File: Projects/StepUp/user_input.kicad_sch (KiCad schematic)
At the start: 1 part, among them U6 COM-09032

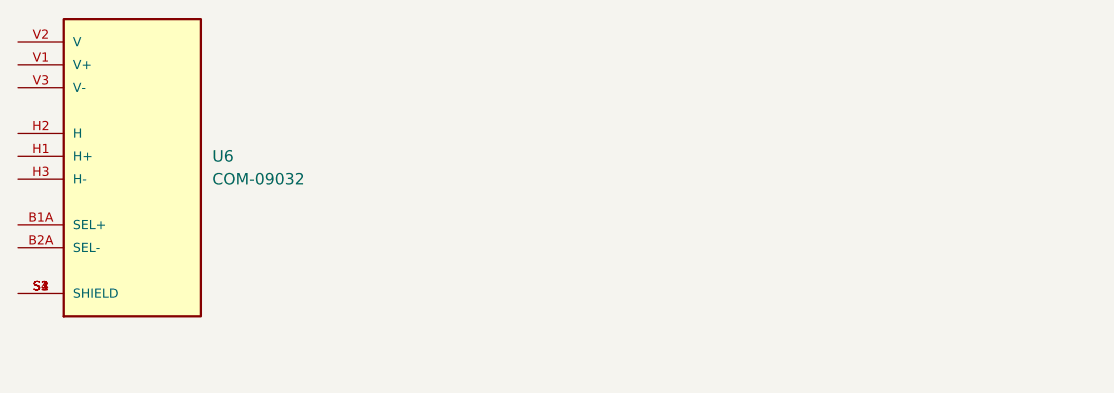
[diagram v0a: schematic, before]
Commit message: feat(charge): Charge IC, USB ESD, sheet sections
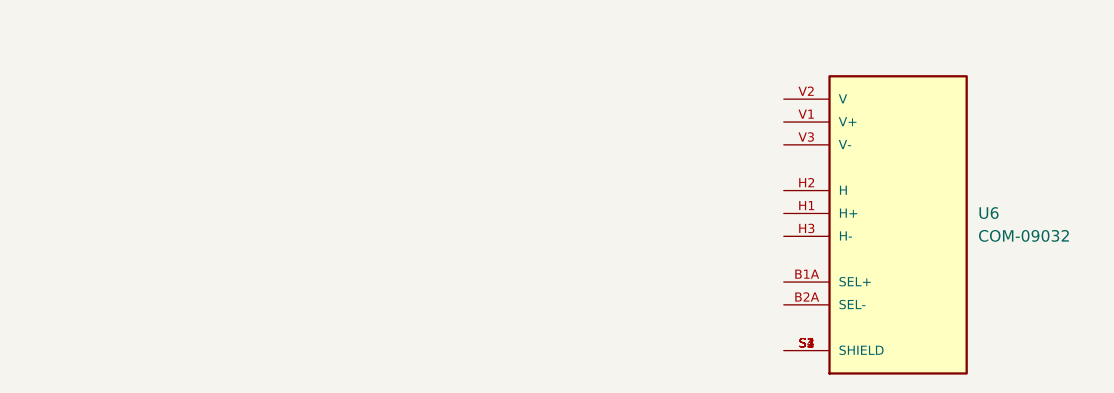
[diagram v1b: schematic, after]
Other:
- moved on the sheet: U6
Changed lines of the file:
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@@
 	(symbol
 		(lib_id "COM-09032:COM-09032")
-		(at 115.57 130.81 0)
+		(at 200.66 137.16 0)
 		(unit 1)
 		(exclude_from_sim no)
@@
 		(fields_autoplaced yes)
 		(property "Reference" "U6"
-			(at 124.46 130.8099 0)
+			(at 209.55 137.1599 0)
 			(effects
 				(font
@@
 		)
 		(property "Value" "COM-09032"
-			(at 124.46 133.3499 0)
+			(at 209.55 139.6999 0)
 			(effects
 				(font
@@
 		)
 		(property "Footprint" "joystick_footprints:XDCR_COM-09032"
-			(at 115.57 130.81 0)
+			(at 200.66 137.16 0)
 			(effects
 				(font
@@
 		)
 		(property "Datasheet" ""
-			(at 115.57 130.81 0)
+			(at 200.66 137.16 0)
 			(effects
 				(font
@@
 		)
 		(property "Description" ""
-			(at 115.57 130.81 0)
+			(at 200.66 137.16 0)
 			(effects
 				(font
@@
 		)
 		(property "MF" "SparkFun Electronics"
-			(at 115.57 130.81 0)
+			(at 200.66 137.16 0)
 			(effects
 				(font
@@
 		)
 		(property "MAXIMUM_PACKAGE_HEIGHT" "30.1mm"
-			(at 115.57 130.81 0)
+			(at 200.66 137.16 0)
 			(effects
 				(font
@@
 		)
 		(property "Package" "Package"
-			(at 115.57 130.81 0)
+			(at 200.66 137.16 0)
 			(effects
 				(font
@@
 		)
 		(property "Price" "None"
-			(at 115.57 130.81 0)
+			(at 200.66 137.16 0)
 			(effects
 				(font
@@
 		)
 		(property "Check_prices" "https://www.snapeda.com/parts/COM-09032/SparkFun+Electronics/view-part/?ref=eda"
-			(at 115.57 130.81 0)
+			(at 200.66 137.16 0)
 			(effects
 				(font
@@
 		)
 		(property "STANDARD" "Manufacturer Recommendations"
-			(at 115.57 130.81 0)
+			(at 200.66 137.16 0)
 			(effects
 				(font
@@
 		)
 		(property "PARTREV" "N/A"
-			(at 115.57 130.81 0)
+			(at 200.66 137.16 0)
 			(effects
 				(font
@@
 		)
 		(property "SnapEDA_Link" "https://www.snapeda.com/parts/COM-09032/SparkFun+Electronics/view-part/?ref=snap"
-			(at 115.57 130.81 0)
+			(at 200.66 137.16 0)
 			(effects
 				(font
@@
 		)
 		(property "MP" "COM-09032"
-			(at 115.57 130.81 0)
+			(at 200.66 137.16 0)
 			(effects
 				(font
@@
 		)
 		(property "Purchase-URL" "https://www.snapeda.com/api/url_track_click_mouser/?unipart_id=888157&manufacturer=SparkFun Electronics&part_name=COM-09032&search_term=joystick"
-			(at 115.57 130.81 0)
+			(at 200.66 137.16 0)
 			(effects
 				(font
@@
 		)
 		(property "Description_1" "\nJoystick, 2 - Axis Analog (Resistive) Output\n"
-			(at 115.57 130.81 0)
+			(at 200.66 137.16 0)
 			(effects
 				(font
@@
 		)
 		(property "Availability" "In Stock"
-			(at 115.57 130.81 0)
+			(at 200.66 137.16 0)
 			(effects
 				(font
@@
 		)
 		(property "MANUFACTURER" "SparkFun Electronics"
-			(at 115.57 130.81 0)
+			(at 200.66 137.16 0)
 			(effects
 				(font
